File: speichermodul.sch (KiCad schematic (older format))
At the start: 65 parts, among them IC1 6116, P1 CONN_3X2, P2 CONN_01X01, P3 CONN_01X01, P4 CONN_01X01, P5 CONN_01X01, P6 CONN_01X01, P7 CONN_01X01, P8 CONN_02X10, P9 CONN_02X10, SW1 SW_PUSH, SW2 SW_PUSH, U1 7400, U2 74LS08, U3 74LS08, U4 74LS14, U5 74LS540, U6 74LS540

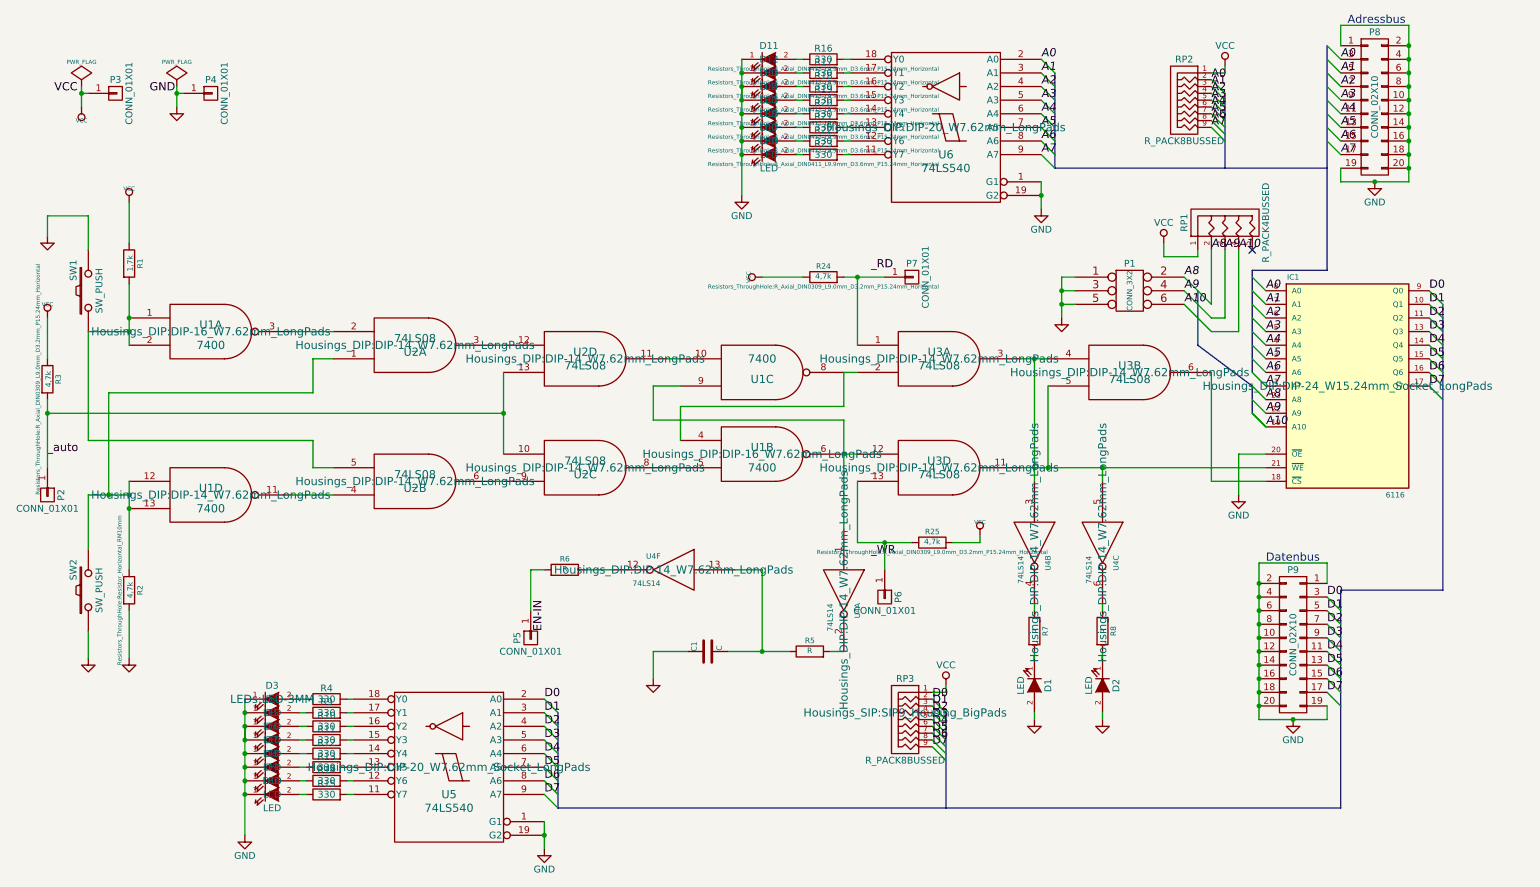
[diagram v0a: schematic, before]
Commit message: einige Leds und Resistoren hinzugefügt und ausgebessert
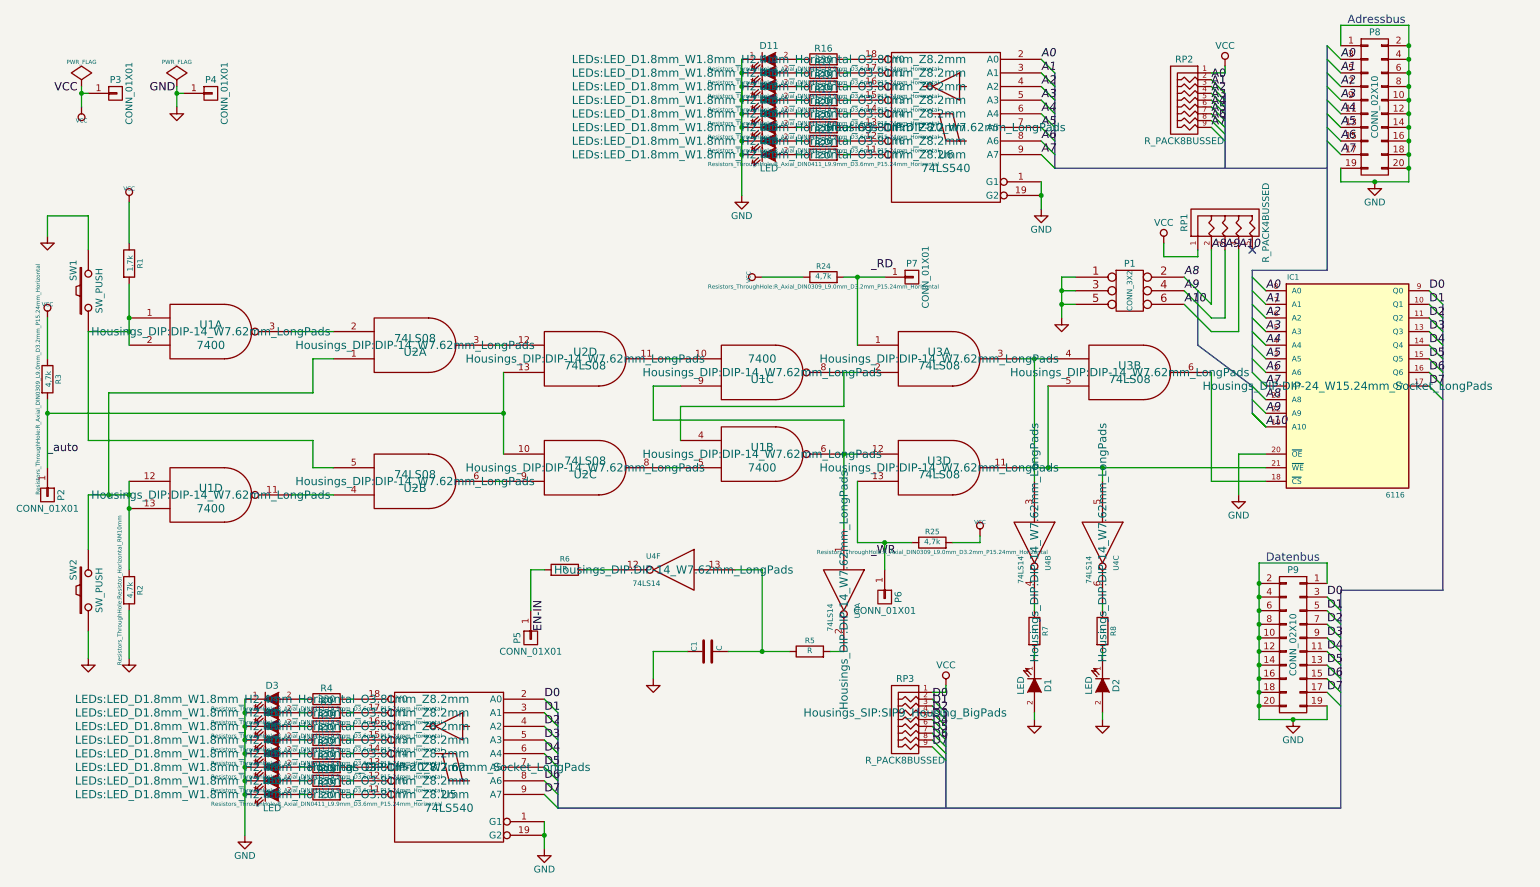
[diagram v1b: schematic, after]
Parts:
- D10, D11, D12, D13, D14, D15, D16, D17, D18, D4, D5, D6, D7, D8, D9: footprint (none) -> LEDs:LED_D1.8mm_W1.8mm_H2.4mm_Horizontal_O3.81mm_Z8.2mm
- D3: footprint LEDs:LED-3MM -> LEDs:LED_D1.8mm_W1.8mm_H2.4mm_Horizontal_O3.81mm_Z8.2mm
- R10, R11, R12, R13, R14, R15, R4, R9: footprint (none) -> Resistors_ThroughHole:R_Axial_DIN0411_L9.9mm_D3.6mm_P15.24mm_Horizontal
- U1: footprint Housings_DIP:DIP-16_W7.62mm_LongPads -> Housings_DIP:DIP-14_W7.62mm_LongPads
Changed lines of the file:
@@
 F 0 "U1" H 1900 3000 60  0000 C CNN
 F 1 "7400" H 1900 2850 60  0000 C CNN
-F 2 "Housings_DIP:DIP-16_W7.62mm_LongPads" H 1900 2950 60  0000 C CNN
+F 2 "Housings_DIP:DIP-14_W7.62mm_LongPads" H 1900 2950 60  0000 C CNN
 F 3 "~" H 1900 2950 60  0000 C CNN
 	1    1900 2950
@@
 F 0 "U1" H 5950 3900 60  0000 C CNN
 F 1 "7400" H 5950 3750 60  0000 C CNN
-F 2 "Housings_DIP:DIP-16_W7.62mm_LongPads" H 5950 3850 60  0000 C CNN
+F 2 "Housings_DIP:DIP-14_W7.62mm_LongPads" H 5950 3850 60  0000 C CNN
 F 3 "~" H 5950 3850 60  0000 C CNN
 	2    5950 3850
@@
 F 0 "U1" H 5950 3300 60  0000 C CNN
 F 1 "7400" H 5950 3150 60  0000 C CNN
-F 2 "Housings_DIP:DIP-16_W7.62mm_LongPads" H 5950 3250 60  0001 C CNN
+F 2 "Housings_DIP:DIP-14_W7.62mm_LongPads" H 5950 3250 60  0000 C CNN
 F 3 "~" H 5950 3250 60  0000 C CNN
 	3    5950 3250
@@
 F 0 "R4" V 2830 5650 50  0000 C CNN
 F 1 "330" V 2750 5650 50  0000 C CNN
-F 2 "" V 2680 5650 30  0001 C CNN
+F 2 "Resistors_ThroughHole:R_Axial_DIN0411_L9.9mm_D3.6mm_P15.24mm_Horizontal" V 2680 5650 30  0000 C CNN
 F 3 "" H 2750 5650 30  0000 C CNN
 	1    2750 5650
@@
 F 0 "R9" V 2830 5750 50  0000 C CNN
 F 1 "330" V 2750 5750 50  0000 C CNN
-F 2 "" V 2680 5750 30  0001 C CNN
+F 2 "Resistors_ThroughHole:R_Axial_DIN0411_L9.9mm_D3.6mm_P15.24mm_Horizontal" V 2680 5750 30  0000 C CNN
 F 3 "" H 2750 5750 30  0000 C CNN
 	1    2750 5750
@@
 F 0 "R10" V 2830 5850 50  0000 C CNN
 F 1 "330" V 2750 5850 50  0000 C CNN
-F 2 "" V 2680 5850 30  0001 C CNN
+F 2 "Resistors_ThroughHole:R_Axial_DIN0411_L9.9mm_D3.6mm_P15.24mm_Horizontal" V 2680 5850 30  0000 C CNN
 F 3 "" H 2750 5850 30  0000 C CNN
 	1    2750 5850
@@
 F 0 "R11" V 2830 5950 50  0000 C CNN
 F 1 "330" V 2750 5950 50  0000 C CNN
-F 2 "" V 2680 5950 30  0001 C CNN
+F 2 "Resistors_ThroughHole:R_Axial_DIN0411_L9.9mm_D3.6mm_P15.24mm_Horizontal" V 2680 5950 30  0000 C CNN
 F 3 "" H 2750 5950 30  0000 C CNN
 	1    2750 5950
@@
 F 0 "R12" V 2830 6050 50  0000 C CNN
 F 1 "330" V 2750 6050 50  0000 C CNN
-F 2 "" V 2680 6050 30  0001 C CNN
+F 2 "Resistors_ThroughHole:R_Axial_DIN0411_L9.9mm_D3.6mm_P15.24mm_Horizontal" V 2680 6050 30  0000 C CNN
 F 3 "" H 2750 6050 30  0000 C CNN
 	1    2750 6050
@@
 F 0 "R13" V 2830 6150 50  0000 C CNN
 F 1 "330" V 2750 6150 50  0000 C CNN
-F 2 "" V 2680 6150 30  0001 C CNN
+F 2 "Resistors_ThroughHole:R_Axial_DIN0411_L9.9mm_D3.6mm_P15.24mm_Horizontal" V 2680 6150 30  0000 C CNN
 F 3 "" H 2750 6150 30  0000 C CNN
 	1    2750 6150
@@
 F 0 "R14" V 2830 6250 50  0000 C CNN
 F 1 "330" V 2750 6250 50  0000 C CNN
-F 2 "" V 2680 6250 30  0001 C CNN
+F 2 "Resistors_ThroughHole:R_Axial_DIN0411_L9.9mm_D3.6mm_P15.24mm_Horizontal" V 2680 6250 30  0000 C CNN
 F 3 "" H 2750 6250 30  0000 C CNN
 	1    2750 6250
@@
 F 0 "R15" V 2830 6350 50  0000 C CNN
 F 1 "330" V 2750 6350 50  0000 C CNN
-F 2 "" V 2680 6350 30  0001 C CNN
+F 2 "Resistors_ThroughHole:R_Axial_DIN0411_L9.9mm_D3.6mm_P15.24mm_Horizontal" V 2680 6350 30  0000 C CNN
 F 3 "" H 2750 6350 30  0000 C CNN
 	1    2750 6350
@@
 F 0 "D3" H 2350 5750 50  0000 C CNN
 F 1 "LED" H 2350 5550 50  0000 C CNN
-F 2 "LEDs:LED-3MM" H 2350 5650 60  0000 C CNN
+F 2 "LEDs:LED_D1.8mm_W1.8mm_H2.4mm_Horizontal_O3.81mm_Z8.2mm" H 2350 5650 60  0000 C CNN
 F 3 "" H 2350 5650 60  0000 C CNN
 	1    2350 5650
@@
 F 0 "D4" H 2350 5850 50  0000 C CNN
 F 1 "LED" H 2350 5650 50  0000 C CNN
-F 2 "" H 2350 5750 60  0001 C CNN
+F 2 "LEDs:LED_D1.8mm_W1.8mm_H2.4mm_Horizontal_O3.81mm_Z8.2mm" H 2350 5750 60  0000 C CNN
 F 3 "" H 2350 5750 60  0000 C CNN
 	1    2350 5750
@@
 F 0 "D5" H 2350 5950 50  0000 C CNN
 F 1 "LED" H 2350 5750 50  0000 C CNN
-F 2 "" H 2350 5850 60  0001 C CNN
+F 2 "LEDs:LED_D1.8mm_W1.8mm_H2.4mm_Horizontal_O3.81mm_Z8.2mm" H 2350 5850 60  0000 C CNN
 F 3 "" H 2350 5850 60  0000 C CNN
 	1    2350 5850
@@
 F 0 "D6" H 2350 6050 50  0000 C CNN
 F 1 "LED" H 2350 5850 50  0000 C CNN
-F 2 "" H 2350 5950 60  0001 C CNN
+F 2 "LEDs:LED_D1.8mm_W1.8mm_H2.4mm_Horizontal_O3.81mm_Z8.2mm" H 2350 5950 60  0000 C CNN
 F 3 "" H 2350 5950 60  0000 C CNN
 	1    2350 5950
@@
 F 0 "D7" H 2350 6150 50  0000 C CNN
 F 1 "LED" H 2350 5950 50  0000 C CNN
-F 2 "" H 2350 6050 60  0001 C CNN
+F 2 "LEDs:LED_D1.8mm_W1.8mm_H2.4mm_Horizontal_O3.81mm_Z8.2mm" H 2350 6050 60  0000 C CNN
 F 3 "" H 2350 6050 60  0000 C CNN
 	1    2350 6050
@@
 F 0 "D8" H 2350 6250 50  0000 C CNN
 F 1 "LED" H 2350 6050 50  0000 C CNN
-F 2 "" H 2350 6150 60  0001 C CNN
+F 2 "LEDs:LED_D1.8mm_W1.8mm_H2.4mm_Horizontal_O3.81mm_Z8.2mm" H 2350 6150 60  0000 C CNN
 F 3 "" H 2350 6150 60  0000 C CNN
 	1    2350 6150
@@
 F 0 "D9" H 2350 6350 50  0000 C CNN
 F 1 "LED" H 2350 6150 50  0000 C CNN
-F 2 "" H 2350 6250 60  0001 C CNN
+F 2 "LEDs:LED_D1.8mm_W1.8mm_H2.4mm_Horizontal_O3.81mm_Z8.2mm" H 2350 6250 60  0000 C CNN
 F 3 "" H 2350 6250 60  0000 C CNN
 	1    2350 6250
@@
 F 0 "D10" H 2350 6450 50  0000 C CNN
 F 1 "LED" H 2350 6250 50  0000 C CNN
-F 2 "" H 2350 6350 60  0001 C CNN
+F 2 "LEDs:LED_D1.8mm_W1.8mm_H2.4mm_Horizontal_O3.81mm_Z8.2mm" H 2350 6350 60  0000 C CNN
 F 3 "" H 2350 6350 60  0000 C CNN
 	1    2350 6350
@@
 F 0 "D11" H 6000 1050 50  0000 C CNN
 F 1 "LED" H 6000 850 50  0000 C CNN
-F 2 "" H 6000 950 60  0001 C CNN
+F 2 "LEDs:LED_D1.8mm_W1.8mm_H2.4mm_Horizontal_O3.81mm_Z8.2mm" H 6000 950 60  0000 C CNN
 F 3 "" H 6000 950 60  0000 C CNN
 	1    6000 950
@@
 F 0 "D12" H 6000 1150 50  0000 C CNN
 F 1 "LED" H 6000 950 50  0000 C CNN
-F 2 "" H 6000 1050 60  0001 C CNN
+F 2 "LEDs:LED_D1.8mm_W1.8mm_H2.4mm_Horizontal_O3.81mm_Z8.2mm" H 6000 1050 60  0000 C CNN
 F 3 "" H 6000 1050 60  0000 C CNN
 	1    6000 1050
@@
 F 0 "D13" H 6000 1250 50  0000 C CNN
 F 1 "LED" H 6000 1050 50  0000 C CNN
-F 2 "" H 6000 1150 60  0001 C CNN
+F 2 "LEDs:LED_D1.8mm_W1.8mm_H2.4mm_Horizontal_O3.81mm_Z8.2mm" H 6000 1150 60  0000 C CNN
 F 3 "" H 6000 1150 60  0000 C CNN
 	1    6000 1150
@@
 F 0 "D14" H 6000 1350 50  0000 C CNN
 F 1 "LED" H 6000 1150 50  0000 C CNN
-F 2 "" H 6000 1250 60  0001 C CNN
+F 2 "LEDs:LED_D1.8mm_W1.8mm_H2.4mm_Horizontal_O3.81mm_Z8.2mm" H 6000 1250 60  0000 C CNN
 F 3 "" H 6000 1250 60  0000 C CNN
 	1    6000 1250
@@
 F 0 "D15" H 6000 1450 50  0000 C CNN
 F 1 "LED" H 6000 1250 50  0000 C CNN
-F 2 "" H 6000 1350 60  0001 C CNN
+F 2 "LEDs:LED_D1.8mm_W1.8mm_H2.4mm_Horizontal_O3.81mm_Z8.2mm" H 6000 1350 60  0000 C CNN
 F 3 "" H 6000 1350 60  0000 C CNN
 	1    6000 1350
@@
 F 0 "D16" H 6000 1550 50  0000 C CNN
 F 1 "LED" H 6000 1350 50  0000 C CNN
-F 2 "" H 6000 1450 60  0001 C CNN
+F 2 "LEDs:LED_D1.8mm_W1.8mm_H2.4mm_Horizontal_O3.81mm_Z8.2mm" H 6000 1450 60  0000 C CNN
 F 3 "" H 6000 1450 60  0000 C CNN
 	1    6000 1450
@@
 F 0 "D17" H 6000 1650 50  0000 C CNN
 F 1 "LED" H 6000 1450 50  0000 C CNN
-F 2 "" H 6000 1550 60  0001 C CNN
+F 2 "LEDs:LED_D1.8mm_W1.8mm_H2.4mm_Horizontal_O3.81mm_Z8.2mm" H 6000 1550 60  0000 C CNN
 F 3 "" H 6000 1550 60  0000 C CNN
 	1    6000 1550
@@
 F 0 "D18" H 6000 1750 50  0000 C CNN
 F 1 "LED" H 6000 1550 50  0000 C CNN
-F 2 "" H 6000 1650 60  0001 C CNN
+F 2 "LEDs:LED_D1.8mm_W1.8mm_H2.4mm_Horizontal_O3.81mm_Z8.2mm" H 6000 1650 60  0000 C CNN
 F 3 "" H 6000 1650 60  0000 C CNN
 	1    6000 1650
